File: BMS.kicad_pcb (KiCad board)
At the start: 2 copper layers, 78 parts, among them J1 Screw_Terminal_01x02, J5 BATT_PACK -, J6 PACK _PACK -, Q22 CSD19531Q5A, Q23 CSD19531Q5A, Q24 CSD19531Q5A, T3 EE20_10_6_750811647, U1 TL431DBZ, U18 VIPer26LD, U2 PC817, U21 BQ7790500PWR, U3 LM3914N

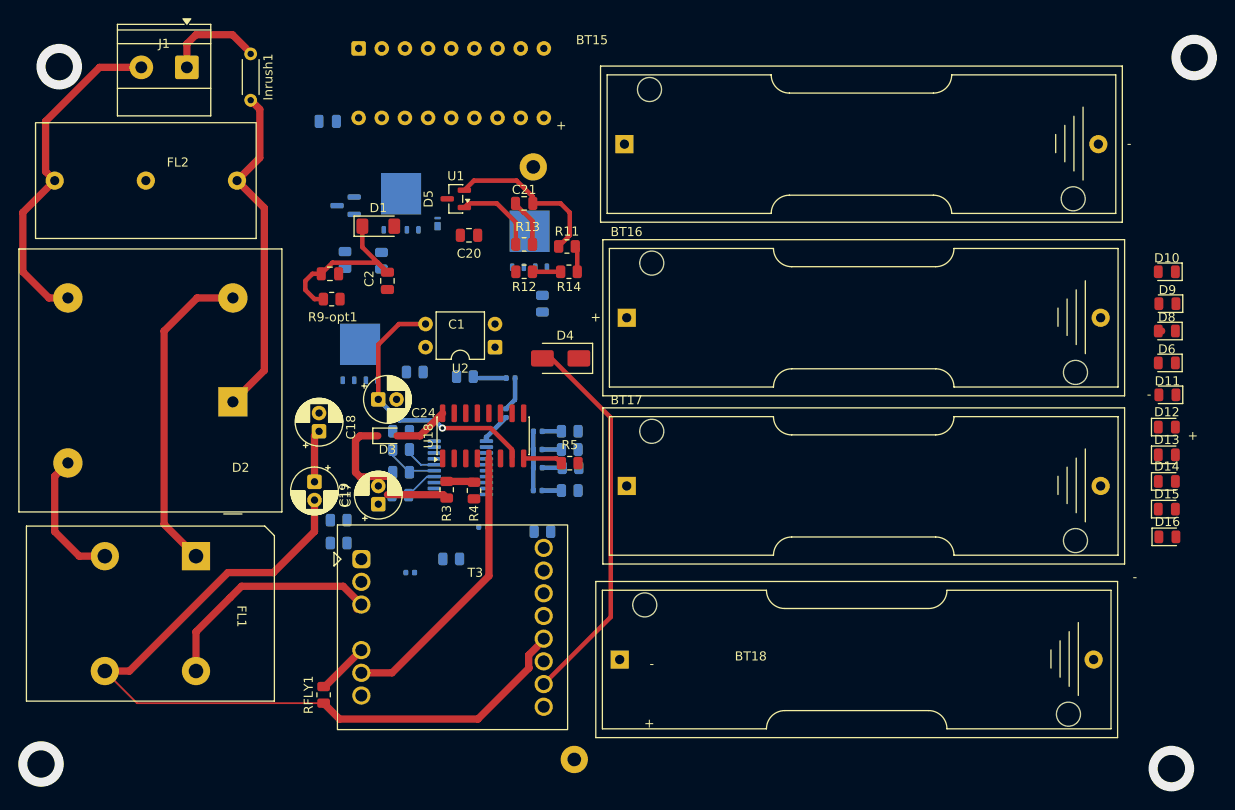
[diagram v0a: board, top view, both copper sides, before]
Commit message: Routing update
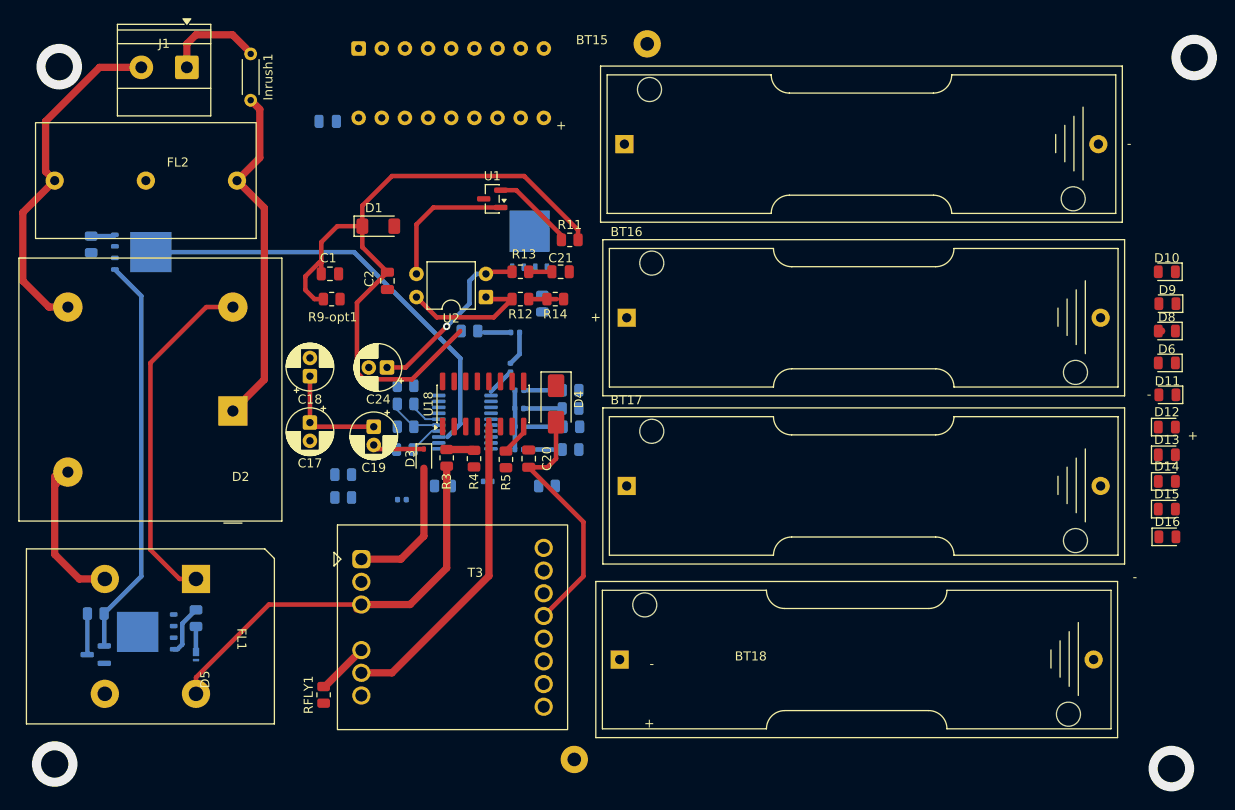
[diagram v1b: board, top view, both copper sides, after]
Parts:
- moved D7 56.4 mm to (106.0, 110.0)
- moved Q24 54.6 mm to (111.7, 107.5), turned to 180 degrees
- moved D5 54.2 mm to (117.0, 110.0), turned to -90 degrees
- moved 1M3 47.5 mm to (106.0, 105.5), turned to 180 degrees
- moved R2 44.2 mm to (117.0, 106.0)
- moved R6 38.2 mm to (105.5, 65.0), turned to -90 degrees
- moved Q23 26.5 mm to (111.0, 65.8), turned to 0 degrees
- moved C20 25.4 mm to (153.5, 88.5), turned to -90 degrees
- moved J5 18.4 mm to (166.5, 43.0)
- moved C19 8.51 mm to (136.5, 85.0), turned to -90 degrees
- moved C21 8.50 mm to (157.0, 68.0)
- moved 6ohm1 8.05 mm to (144.1, 91.5)
- moved C37 8.05 mm to (139.6, 93.0)
- moved R5 7.01 mm to (151.0, 88.6), turned to -90 degrees
- moved C17 6.52 mm to (129.5, 84.5)
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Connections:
- 1M5 pad 2: V- -> PACK-
- 6ohm1 pad 2: Net-(J5-Pin_1) -> PACK-
- C20 pad 1: (no net) -> Net-(C20-Pad1)
- C20 pad 2: (no net) -> Net-(D4-A)
- D5 pad 2: V- -> PACK-
- J5 pad 1: Net-(J5-Pin_1) -> PACK-
- Q24 pad 5: V- -> PACK-
- Rsrn1 pad 2: Net-(J5-Pin_1) -> PACK-
- U2 pad 1: Net-(R12-Pad2) -> VDD_U18
- U2 pad 2: Net-(U1-K) -> FB
- U2 pad 3: FB -> Net-(U1-K)
- U2 pad 4: VDD_U18 -> Net-(R12-Pad2)
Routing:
- net GND: track 93.1 -> 6.52 mm, vias 0 -> 4
- net VO: track 26.5 -> 82.3 mm
- net CHG: track 0.00 -> 48.0 mm
- net Net-(D7-A): track 0.00 -> 44.2 mm
- net Net-(C17-Pad1): track 38.4 -> 58.4 mm
- net Net-(R12-Pad2): track 0.00 -> 15.6 mm
- net Net-(D4-A): track 42.5 -> 28.0 mm
- net FB: track 30.1 -> 16.6 mm
- net Net-(D3-A): track 6.03 -> 15.4 mm
- net Net-(U1-K): track 9.11 -> 18.4 mm
- net Net-(U1-REF): track 21.2 -> 12.3 mm
- net Net-(D5-K): track 0.00 -> 7.31 mm
- net Net-(Q24-G): track 0.00 -> 5.58 mm
- net Net-(D3-K): track 9.88 -> 5.69 mm
- net VDD_U18: track 31.3 -> 34.8 mm
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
